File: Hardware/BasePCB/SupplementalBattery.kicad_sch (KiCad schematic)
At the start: 30 parts, among them J1 53307-2471, Q6 IRLML0030

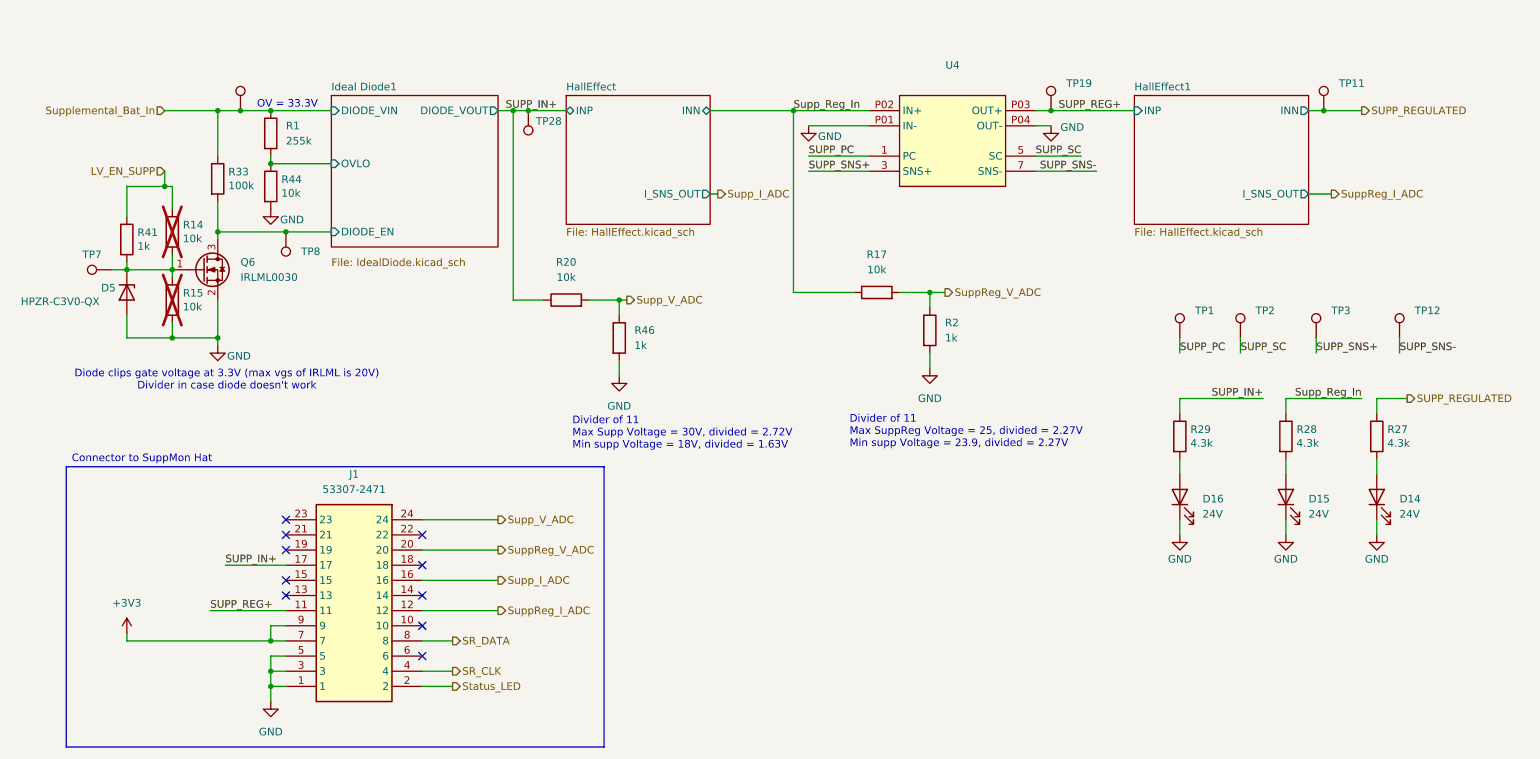
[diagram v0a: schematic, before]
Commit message: updated p/n
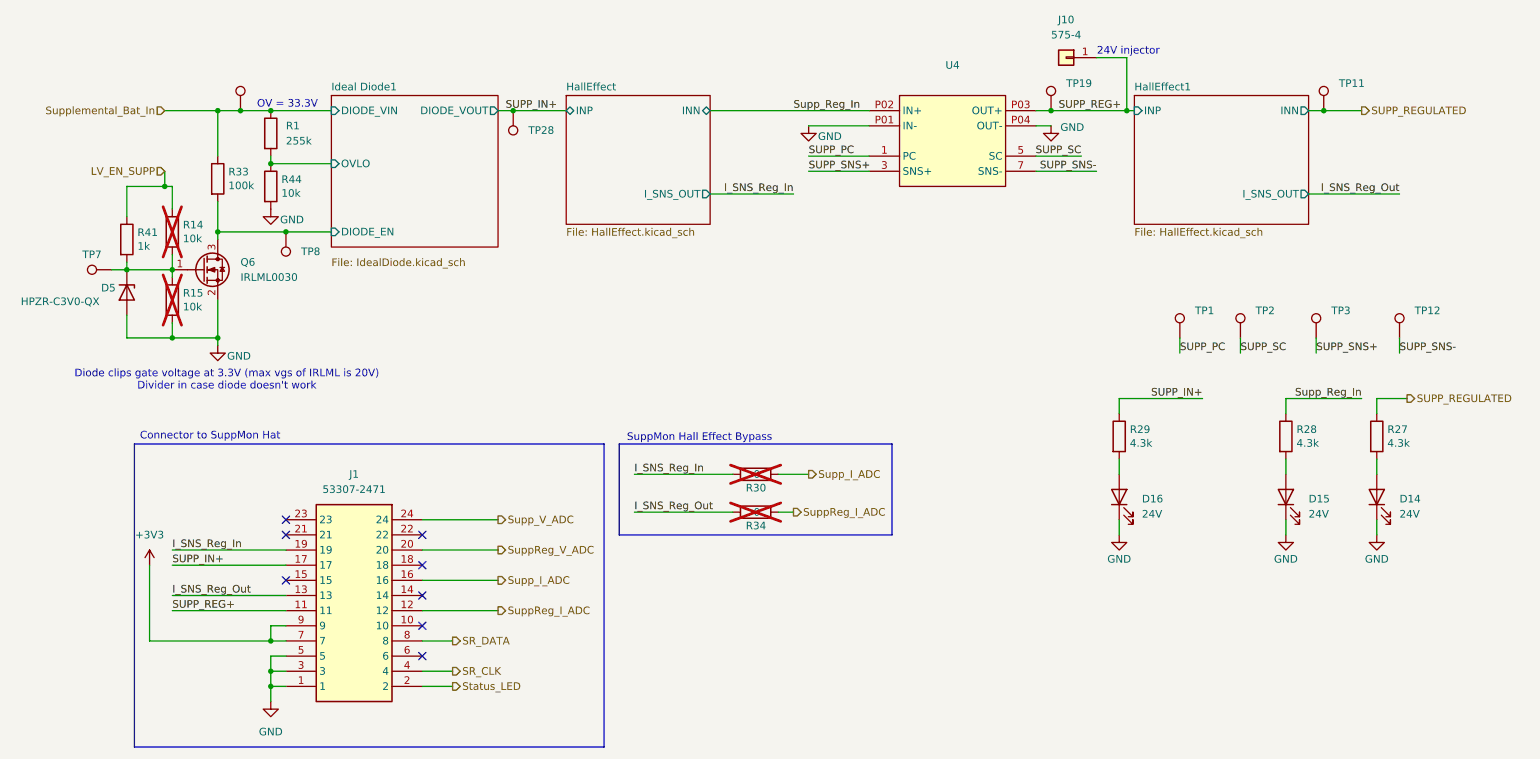
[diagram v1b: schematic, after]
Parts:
- removed R17, R20: 10k, Resistor_SMD:R_0603_1608Metric_Pad0.98x0.95mm_HandSolder, symbol Device:R
- removed R2, R46: 1k, Resistor_SMD:R_0603_1608Metric_Pad0.98x0.95mm_HandSolder, symbol Device:R
- added J10: 575-4, UTSVT_Connectors:5754, symbol Connector_Generic:Conn_01x01
- added R30, R34: 0, Resistor_SMD:R_0603_1608Metric_Pad0.98x0.95mm_HandSolder, symbol Device:R
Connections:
- net SUPP_REG+: now also J10.1 (Pin_1)
- net SuppReg_I_ADC: now also R34.2
- net Supp_I_ADC: now also R30.2
- net I_SNS_Reg_Out: now reaches J1.13
- net I_SNS_Reg_Out: now also R34.1
- net I_SNS_Reg_In: now reaches J1.19
- net I_SNS_Reg_In: now also R30.1
- no-connect marks 10 -> 8
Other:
- note added: "24V injector"
- note added: "SuppMon Hall Effect Bypass"
- note removed: "Divider of 11 Max Supp Voltage = 30V, divided = 2.72V Min supp Voltage = 18V, divided = 1.63V"
- note removed: "Divider of 11 Max SuppReg Voltage = 25, divided = 2.27V Min supp Voltage = 23.9, divided = 2.27V"
- moved on the sheet: D16, R29, TP28
